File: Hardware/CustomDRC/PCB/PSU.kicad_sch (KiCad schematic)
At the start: 0 parts

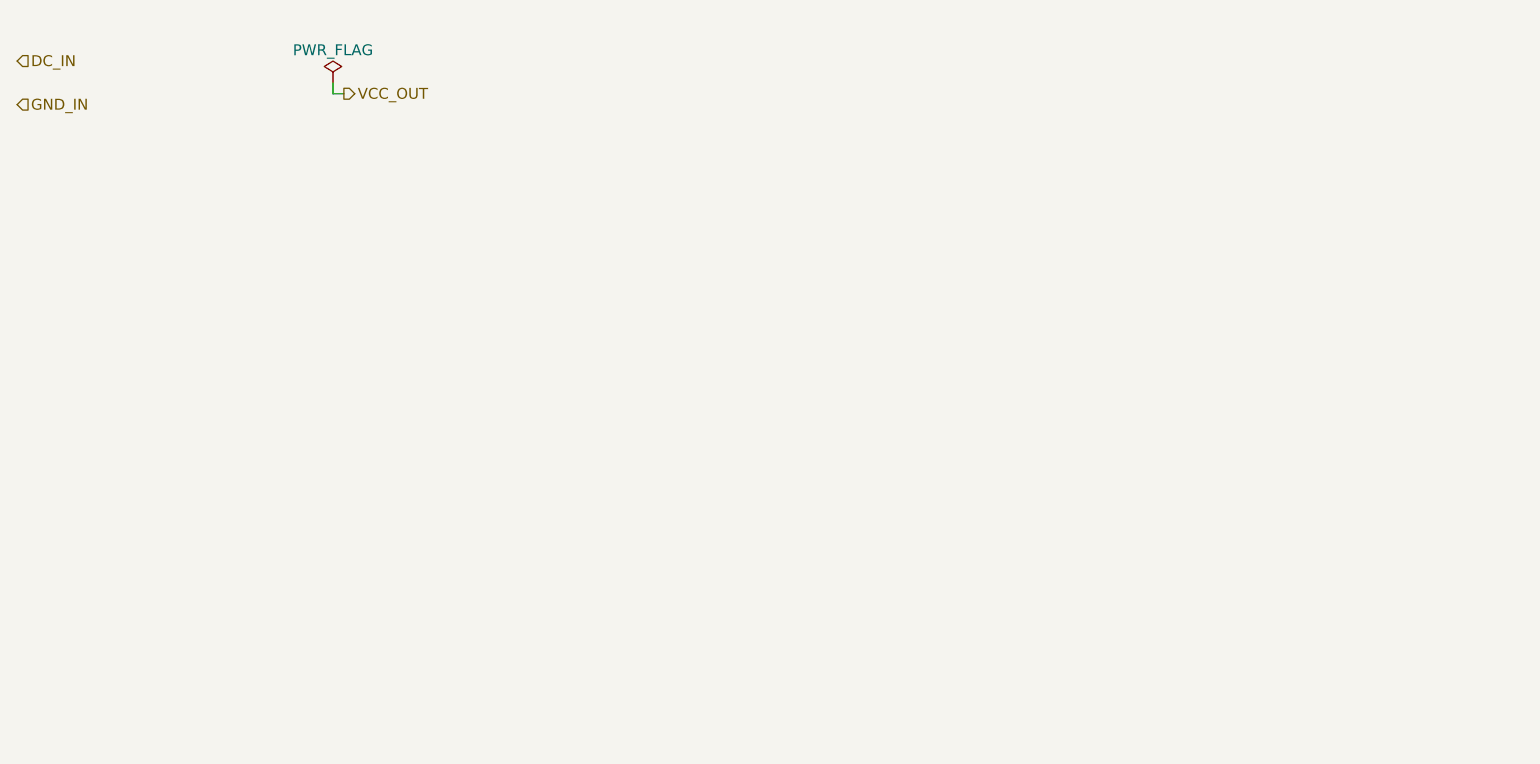
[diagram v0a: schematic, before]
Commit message: Update - finished schematic for revision A
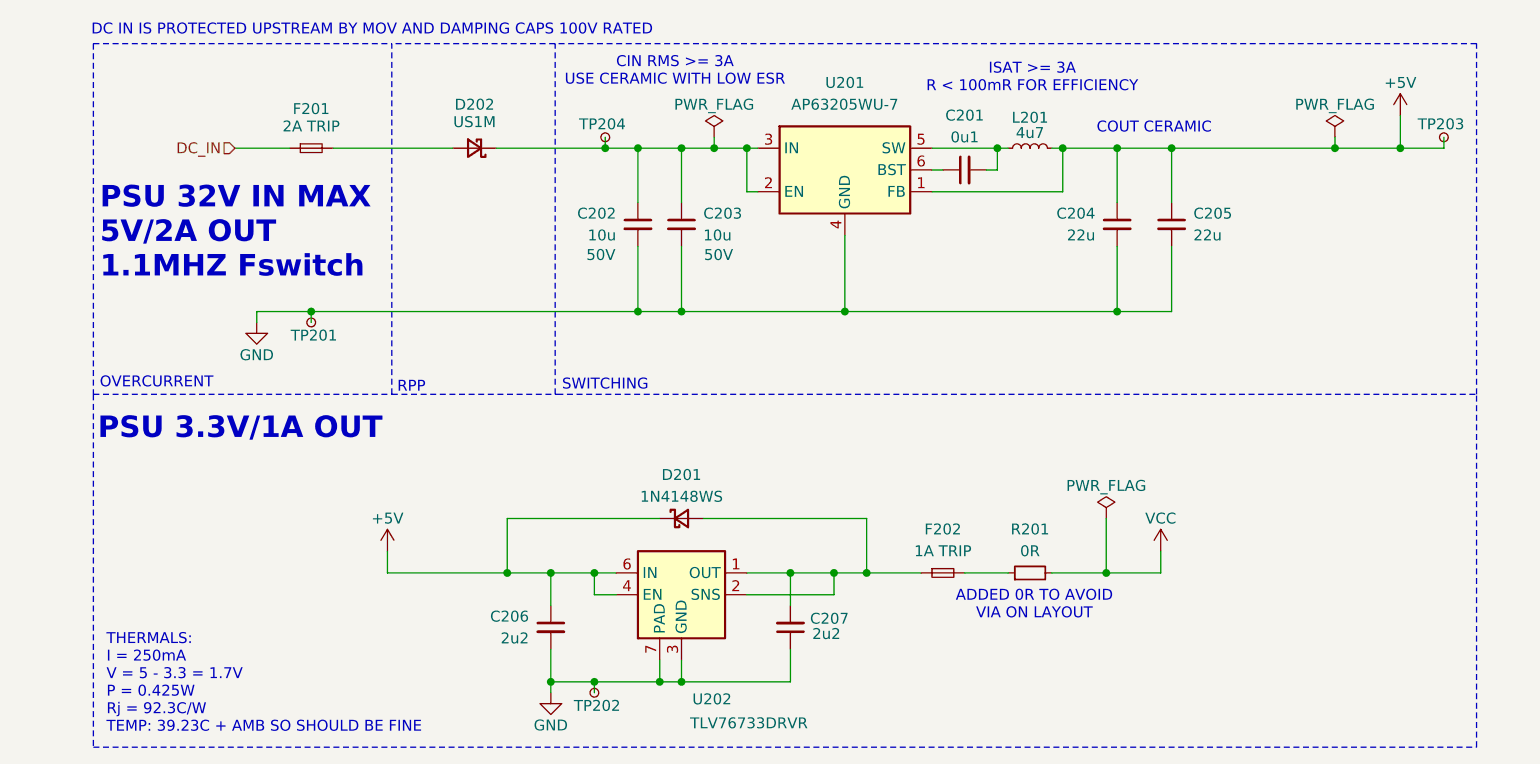
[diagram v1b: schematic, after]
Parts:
- added C201: 0u1, Capacitor_SMD:C_0603_1608Metric_Pad1.08x0.95mm_HandSolder, symbol Device:C_Small
- added C202, C203: 10u, Capacitor_SMD:C_1206_3216Metric_Pad1.33x1.80mm_HandSolder, symbol Device:C_Small
- added C204, C205: 22u, Capacitor_SMD:C_0805_2012Metric_Pad1.18x1.45mm_HandSolder, symbol Device:C_Small
- added C206, C207: 2u2, Capacitor_SMD:C_0805_2012Metric_Pad1.18x1.45mm_HandSolder, symbol Device:C_Small
- added D201: 1N4148WS, Diode_SMD:D_SOD-323_HandSoldering, symbol Device:D_Schottky_Small
- added D202: US1M, Diode_SMD:D_SMA_Handsoldering, symbol Device:D_Schottky_Small
- added F201: 2A TRIP, Fuse:Fuse_1206_3216Metric_Pad1.42x1.75mm_HandSolder, symbol Device:Fuse_Small
- added F202: 1A TRIP, Fuse:Fuse_0603_1608Metric_Pad1.05x0.95mm_HandSolder, symbol Device:Fuse_Small
- added L201: 4u7, Inductor_SMD:L_Chilisin_BMRA00040420, symbol Device:L_Small
- added R201: 0R, Resistor_SMD:R_0603_1608Metric_Pad0.98x0.95mm_HandSolder, symbol Device:R_Small
- added TP201, TP202, TP203, TP204: TestPoint_Small, TestPoint:TestPoint_Pad_D1.5mm, symbol Connector:TestPoint_Small
- added U201: AP63205WU-7, Package_TO_SOT_SMD:TSOT-23-6, symbol Regulator_Switching:AP63205WU
- added U202: TLV76733DRVR, Package_SON:WSON-6-1EP_2x2mm_P0.65mm_EP1x1.6mm_ThermalVias, symbol Regulator_Linear:TLV76733DRVx
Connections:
- net DC_IN: now also F201.1
- new net: C202.1, C203.1, D202.1 (K), TP204.1, U201.2 (EN), U201.3 (IN)
- new net: D202.2 (A), F201.2
- new net: C207.2, D201.2 (A), F202.1, U202.1 (OUT), U202.2 (SNS)
- new net: F202.2, R201.1
- new net: C201.2, L201.1, U201.5 (SW)
- new net: C201.1, U201.6 (BST)
- new net +5V: C204.1, C205.1, C206.1, D201.1 (K), L201.2, TP203.1, U201.1 (FB), U202.4 (EN), U202.6 (IN)
- new net GND: C202.2, C203.2, C204.2, C205.2, C206.2, C207.1, TP201.1, TP202.1, U201.4 (GND), U202.3 (GND), U202.5 (GND), U202.7 (PAD)
- new net VCC: R201.2
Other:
- note added: "ADDED 0R TO AVOID VIA ON LAYOUT"
- note added: "CIN RMS >= 3A USE CERAMIC WITH LOW ESR"
- note added: "COUT CERAMIC"
- note added: "DC IN IS PROTECTED UPSTREAM BY MOV AND DAMPING CAPS 100V RATED"
- note added: "ISAT >= 3A R < 100mR FOR EFFICIENCY"
- note added: "OVERCURRENT"
- note added: "PSU 3.3V/1A OUT"
- note added: "PSU 32V IN MAX 5V/2A OUT 1.1MHZ Fswitch"
- note added: "RPP"
- note added: "SWITCHING"
- note added: "THERMALS: I = 250mA V = 5 - 3.3 = 1.7V P = 0.425W Rj = 92.3C/W TEMP: 39.23C + AMB SO SHOULD BE FINE"
- company: (none) -> JS HW
- title: (none) -> CDRC - Custom DRC for Audison AC Link

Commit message: Sync HW changes for V1 PCB
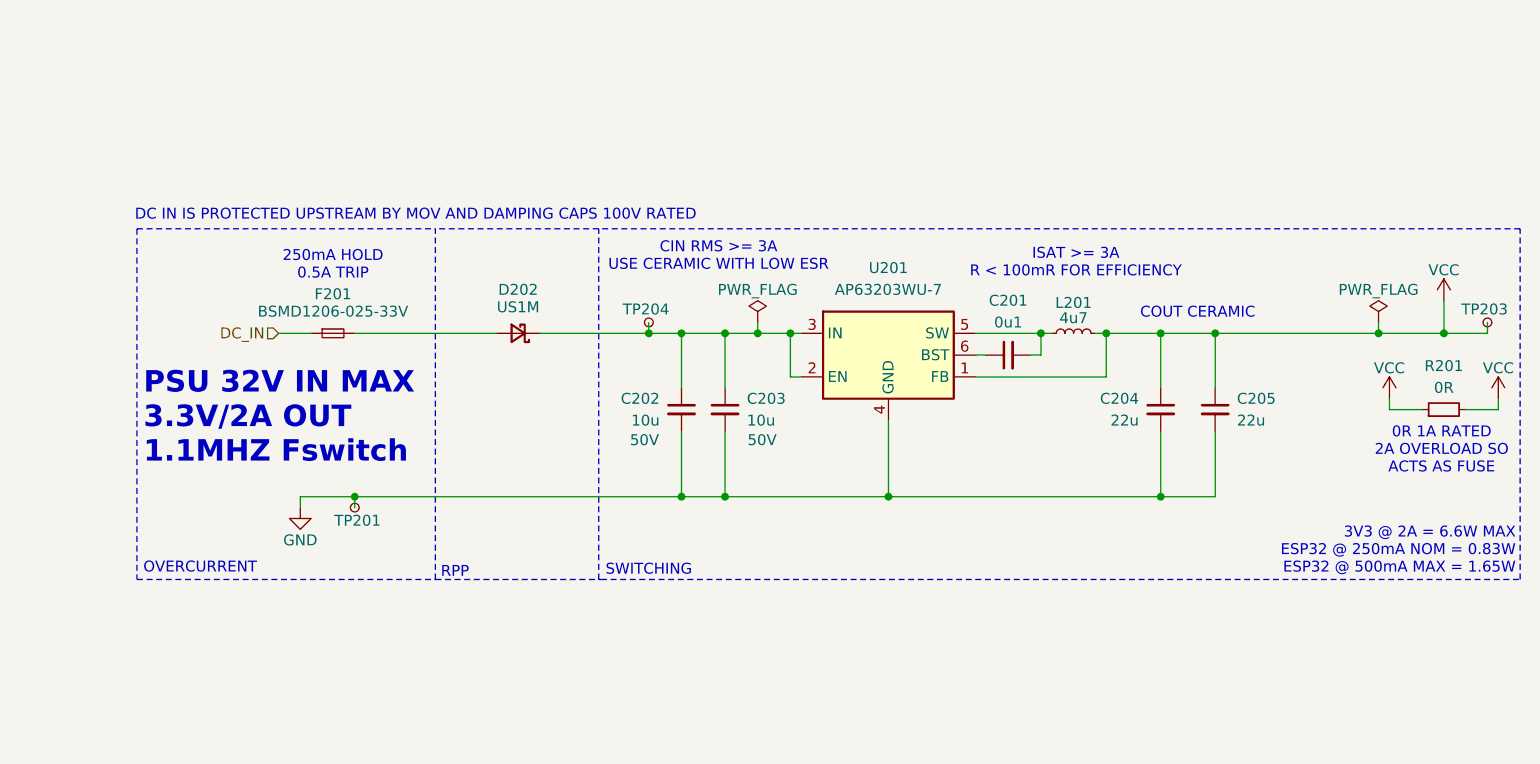
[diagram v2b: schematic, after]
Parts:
- removed C206, C207: 2u2, Capacitor_SMD:C_0805_2012Metric_Pad1.18x1.45mm_HandSolder, symbol Device:C_Small
- removed D201: 1N4148WS, Diode_SMD:D_SOD-323_HandSoldering, symbol Device:D_Schottky_Small
- removed F202: 1A TRIP, Fuse:Fuse_0603_1608Metric_Pad1.05x0.95mm_HandSolder, symbol Device:Fuse_Small
- removed TP202: TestPoint_Small, TestPoint:TestPoint_Pad_D1.5mm, symbol Connector:TestPoint_Small
- removed U202: TLV76733DRVR, Package_SON:WSON-6-1EP_2x2mm_P0.65mm_EP1x1.6mm_ThermalVias, symbol Regulator_Linear:TLV76733DRVx
- F201: value 2A TRIP -> BSMD1206-025-33V
- L201: footprint Inductor_SMD:L_Chilisin_BMRA00040420 -> Inductor_SMD:L_Cenker_CKCS4030; LCSC C5307591 -> C96899; MPN XR0420-4R7M -> SWPA4030S3R9MT; Manufacturer XR -> Sunlord
- U201: value AP63205WU-7 -> AP63203WU-7; LCSC C2071056 -> C780769; MPN AP63205WU-7 -> AP63203WU-7
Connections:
- net +5V is gone; now on net VCC: C204.1, C205.1, L201.2, TP203.1, U201.1 (FB)
- net VCC: now also R201.1
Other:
- note added: "0R 1A RATED 2A OVERLOAD SO ACTS AS FUSE"
- note added: "250mA HOLD 0.5A TRIP"
- note added: "3V3 @ 2A = 6.6W MAX ESP32 @ 250mA NOM = 0.83W ESP32 @ 500mA MAX = 1.65W"
- note added: "PSU 32V IN MAX 3.3V/2A OUT 1.1MHZ Fswitch"
- note removed: "ADDED 0R TO AVOID VIA ON LAYOUT"
- note removed: "PSU 3.3V/1A OUT"
- note removed: "PSU 32V IN MAX 5V/2A OUT 1.1MHZ Fswitch"
- note removed: "THERMALS: I = 250mA V = 5 - 3.3 = 1.7V P = 0.425W Rj = 92.3C/W TEMP: 39.23C + AMB SO SHOULD BE FINE"
- moved on the sheet: C201, C202, C203, C204, C205, D202, F201, L201, TP201, TP203, TP204, U201
